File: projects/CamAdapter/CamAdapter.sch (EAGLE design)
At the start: 4 parts

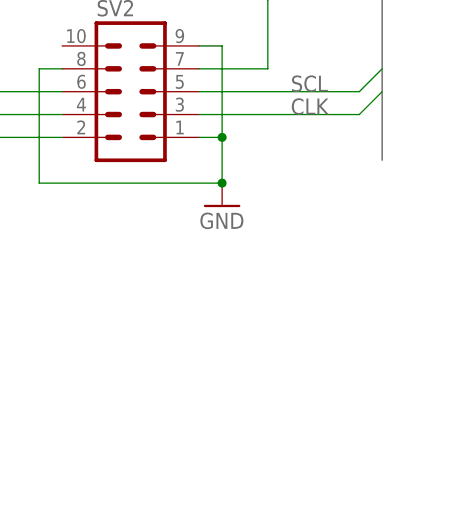
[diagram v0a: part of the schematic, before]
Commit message: pcb2gcode outline & drill test
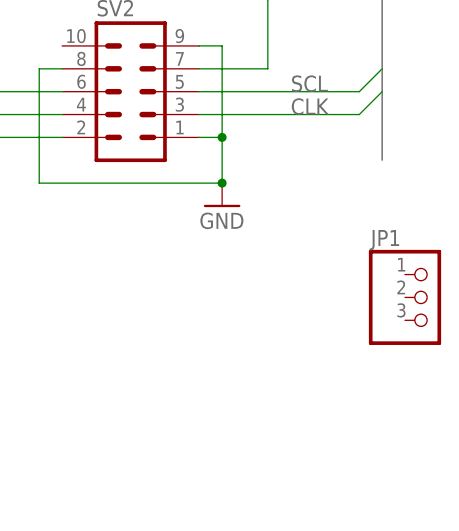
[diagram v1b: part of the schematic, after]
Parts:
- added JP1: (no value), pinhead:PINHD-1X3
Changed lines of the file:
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@@
 <part name="P+3" library="supply1" deviceset="VCC" device=""/>
 <part name="GND3" library="supply1" deviceset="GND" device=""/>
+<part name="JP1" library="pinhead" deviceset="PINHD-1X3" device=""/>
 </parts>
 <sheets>
@@
 <instance part="P+3" gate="VCC" x="60.96" y="93.98"/>
 <instance part="GND3" gate="1" x="60.96" y="71.12"/>
+<instance part="JP1" gate="A" x="167.64" y="91.44"/>
 </instances>
 <busses>

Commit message: Final
* finally found out pcb2gcode and CAM settings so that
  lower right corner is origin and coordinates relative to that point
	lign up when CNC milling
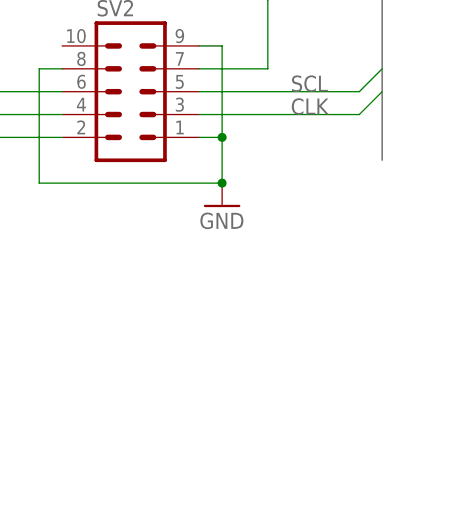
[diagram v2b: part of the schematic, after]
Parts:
- removed JP1: (no value), pinhead:PINHD-1X3
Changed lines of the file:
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@@
 <part name="P+3" library="supply1" deviceset="VCC" device=""/>
 <part name="GND3" library="supply1" deviceset="GND" device=""/>
-<part name="JP1" library="pinhead" deviceset="PINHD-1X3" device=""/>
 </parts>
 <sheets>
@@
 <instance part="P+3" gate="VCC" x="60.96" y="93.98"/>
 <instance part="GND3" gate="1" x="60.96" y="71.12"/>
-<instance part="JP1" gate="A" x="167.64" y="91.44"/>
 </instances>
 <busses>
